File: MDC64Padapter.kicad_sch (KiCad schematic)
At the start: 34 parts, among them J1 DB9_F_TO_C64, J2 DB9_M_TO_PAD, Q1 BC847, Q2 BC847, SW1 MODE, U1 74ACT08, U2 74ACT373, U3 74ACT157, U4 74ACT373, U5 74AHC1G04, U6 NE555D

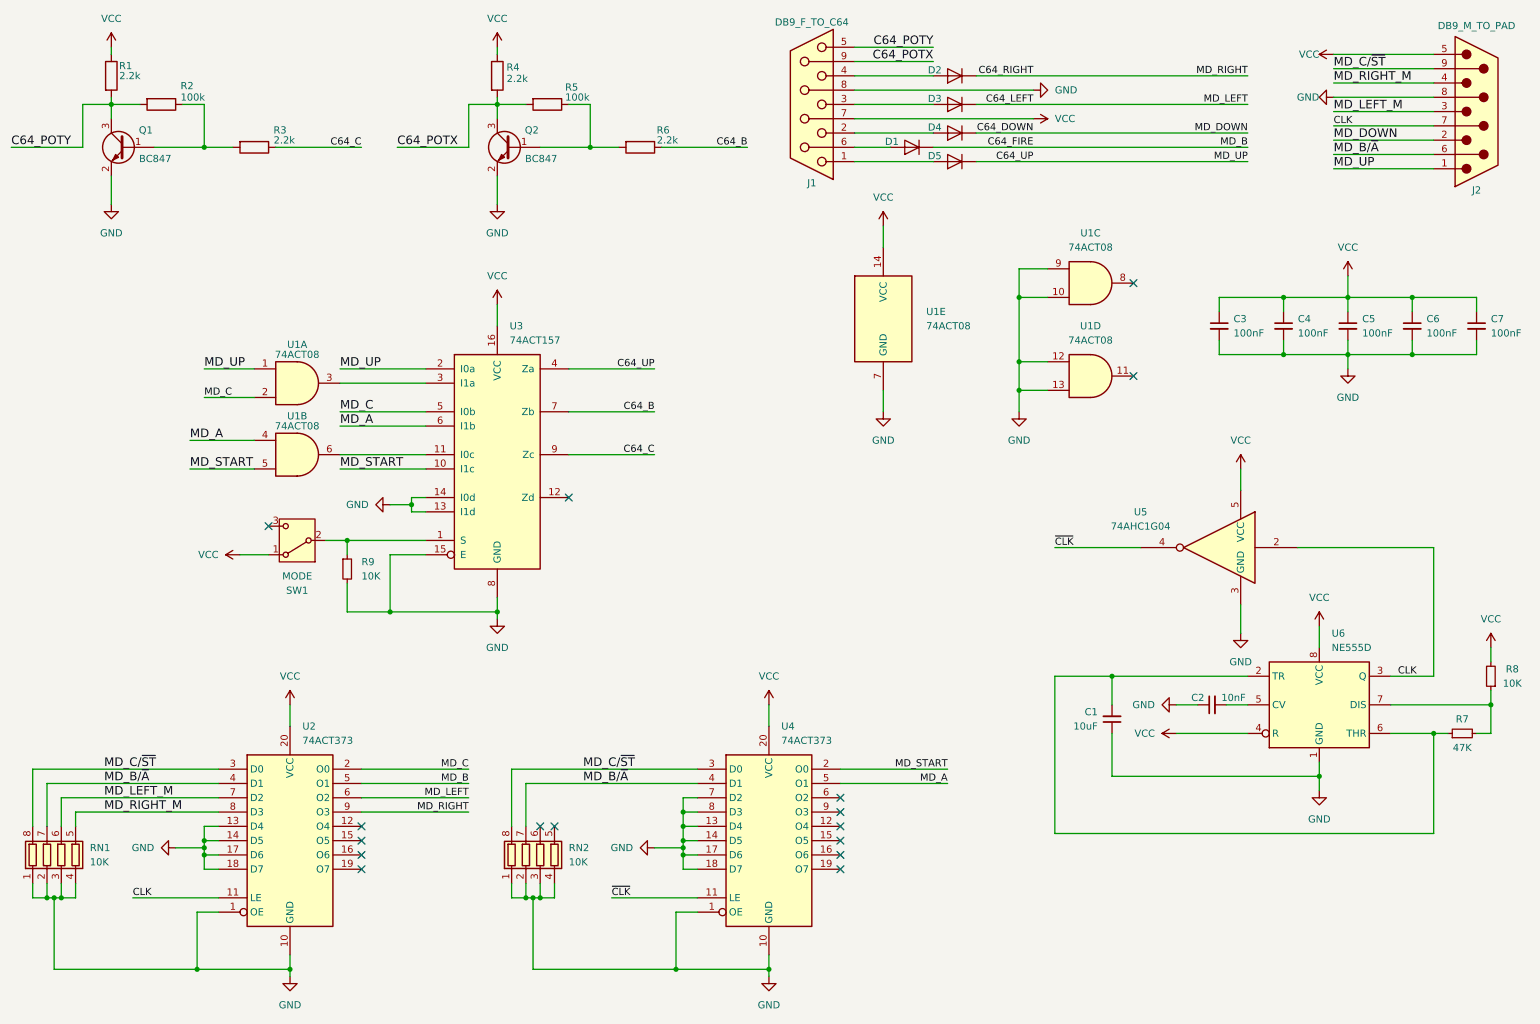
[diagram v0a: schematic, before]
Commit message: Reorganize pcb a bit
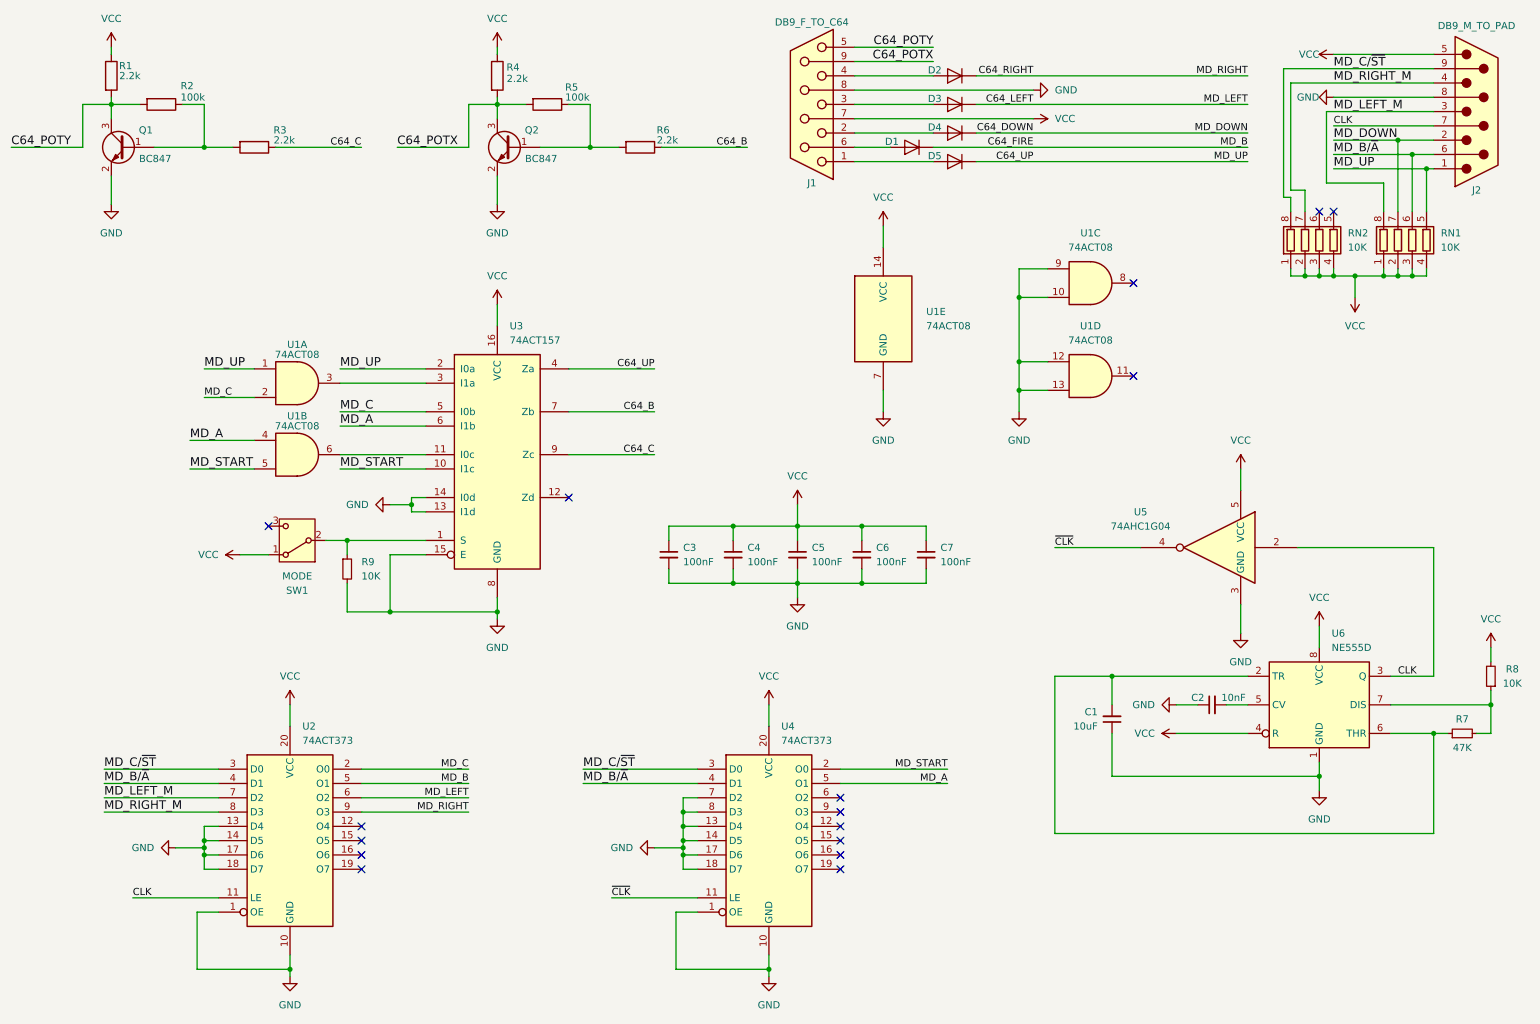
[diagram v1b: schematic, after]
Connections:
- net C64_DOWN: now also RN1.7 (R2.2)
- net C64_UP: now also RN1.5 (R4.2)
- net GND: no longer RN1.1 (R1.1), RN1.2 (R2.1), RN1.3 (R3.1), RN1.4 (R4.1), RN2.1 (R1.1), RN2.2 (R2.1), RN2.3 (R3.1), RN2.4 (R4.1)
- net MD_B/~{A}: now also RN1.6 (R3.2); no longer RN1.7 (R2.2), RN2.7 (R2.2)
- net MD_C/~{ST}: no longer RN1.8 (R1.2)
- net MD_LEFT_M: now also RN1.8 (R1.2); no longer RN1.6 (R3.2)
- net MD_RIGHT_M: now also RN2.7 (R2.2); no longer RN1.5 (R4.2)
- net VCC: now also RN1.1 (R1.1), RN1.2 (R2.1), RN1.3 (R3.1), RN1.4 (R4.1), RN2.1 (R1.1), RN2.2 (R2.1), RN2.3 (R3.1), RN2.4 (R4.1)
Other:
- moved on the sheet: C3, C4, C5, C6, C7, RN1, RN2
